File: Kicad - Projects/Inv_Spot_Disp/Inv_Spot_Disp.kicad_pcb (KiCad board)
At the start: 2 copper layers, 128.6 x 75.3 mm, 39 parts, among them J1 PWM_Out, J2 Power_Supply, J3 Trigger, J4 Prog, SW1 1, SW2 2, SW3 3, SW4 4, SW5 SW_Push, U1 STM32F030F4Px, U2 NHD-0420H1Z, U3 AMS1117-3.3, U4 LKS561, U5 L7805, U6 LTV-817S

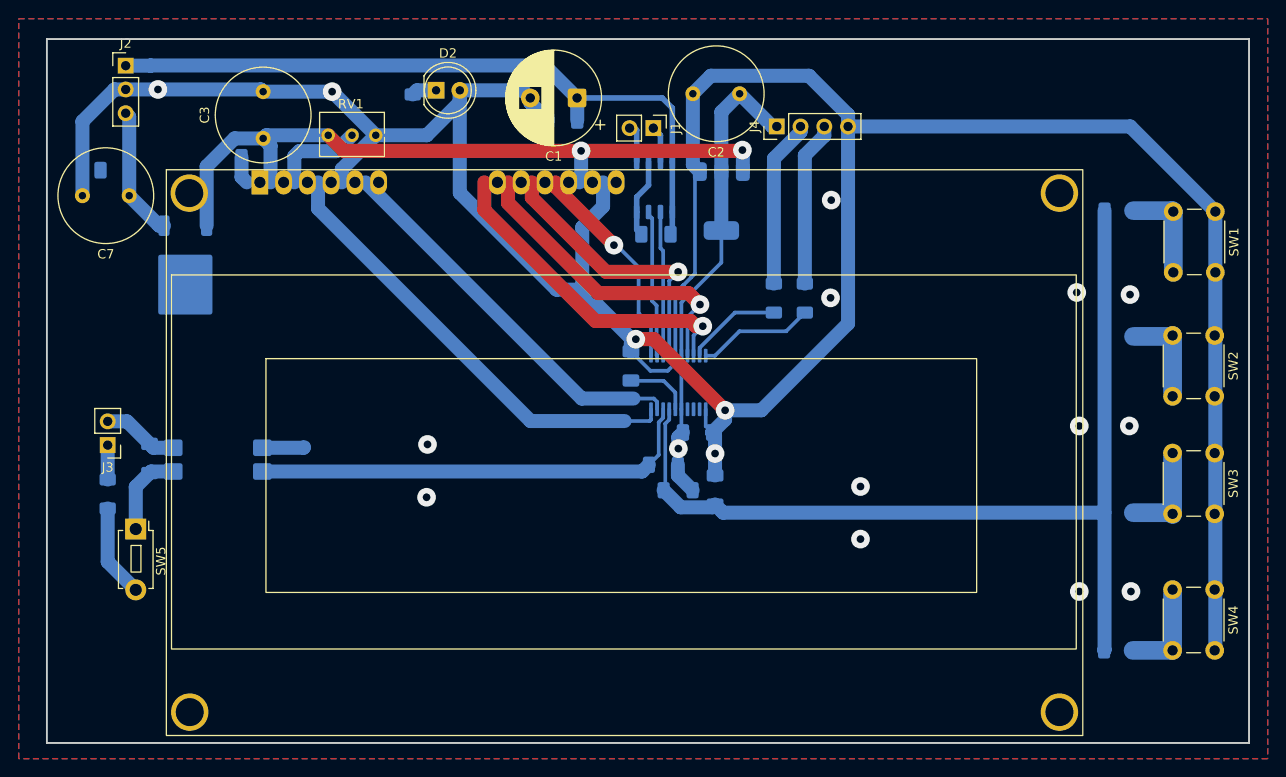
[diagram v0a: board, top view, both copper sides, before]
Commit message: Cotações
Cotações
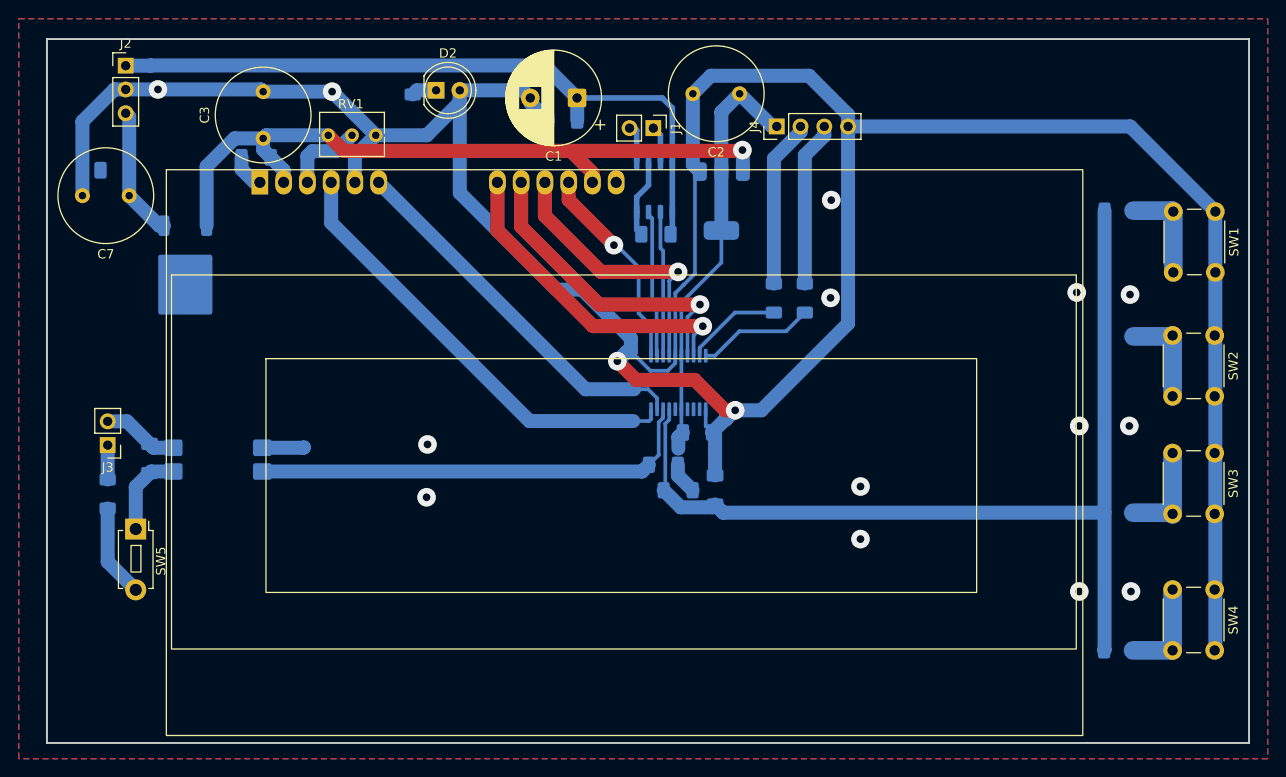
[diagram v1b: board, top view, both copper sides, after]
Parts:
- removed C12: 104, Capacitor_SMD:C_1206_3216Metric_Pad1.33x1.80mm_HandSolder
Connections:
- U1 pad 6: Current_Sense -> unconnected-(U1-PA0-Pad6)
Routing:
- net GND: track 346.7 -> 336.0 mm, vias 17 -> 16
- net Current_Sense: track 7.07 -> 0.00 mm
- net 5V: track 76.5 -> 78.0 mm, vias 2 -> 1
- net Net-(U2-VO): track 9.90 -> 8.50 mm
- net Enable: track 41.7 -> 40.5 mm
- net D7: track 22.9 -> 22.3 mm
- net RS: track 49.0 -> 48.5 mm
- net 3V3: vias 1 -> 0
